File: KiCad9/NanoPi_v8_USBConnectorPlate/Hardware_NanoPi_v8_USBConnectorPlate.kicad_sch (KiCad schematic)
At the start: 30 parts, among them J1 Conn_01x02, J10 Conn_01x04, J11 Conn_01x02, J12 Conn_01x02, J2 USB_Host_Data_02x02, J3 USB_Host_Data_02x02, J4 USB_Power_02x02, J5 Conn_01x03, J6 Conn_01x09, J8 Conn_01x09, U1 USBLC6-2P6, U2 USBLC6-2P6, U3 USBLC6-2P6

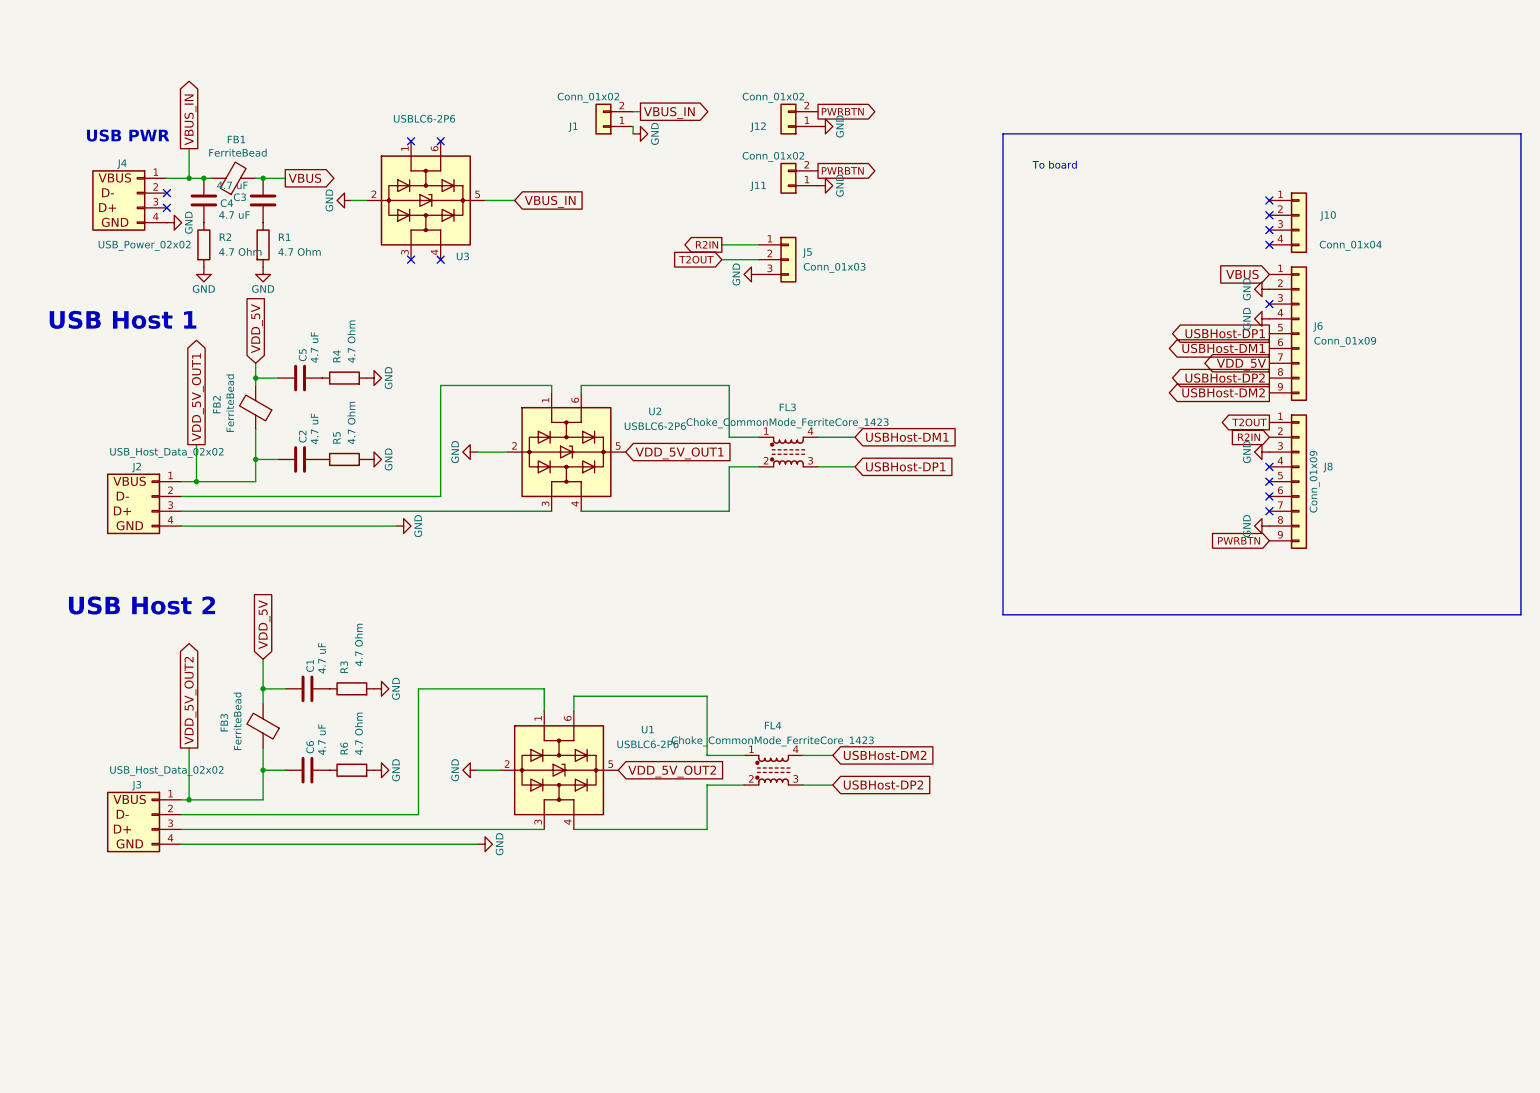
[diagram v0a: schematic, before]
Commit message: add ethernet etc
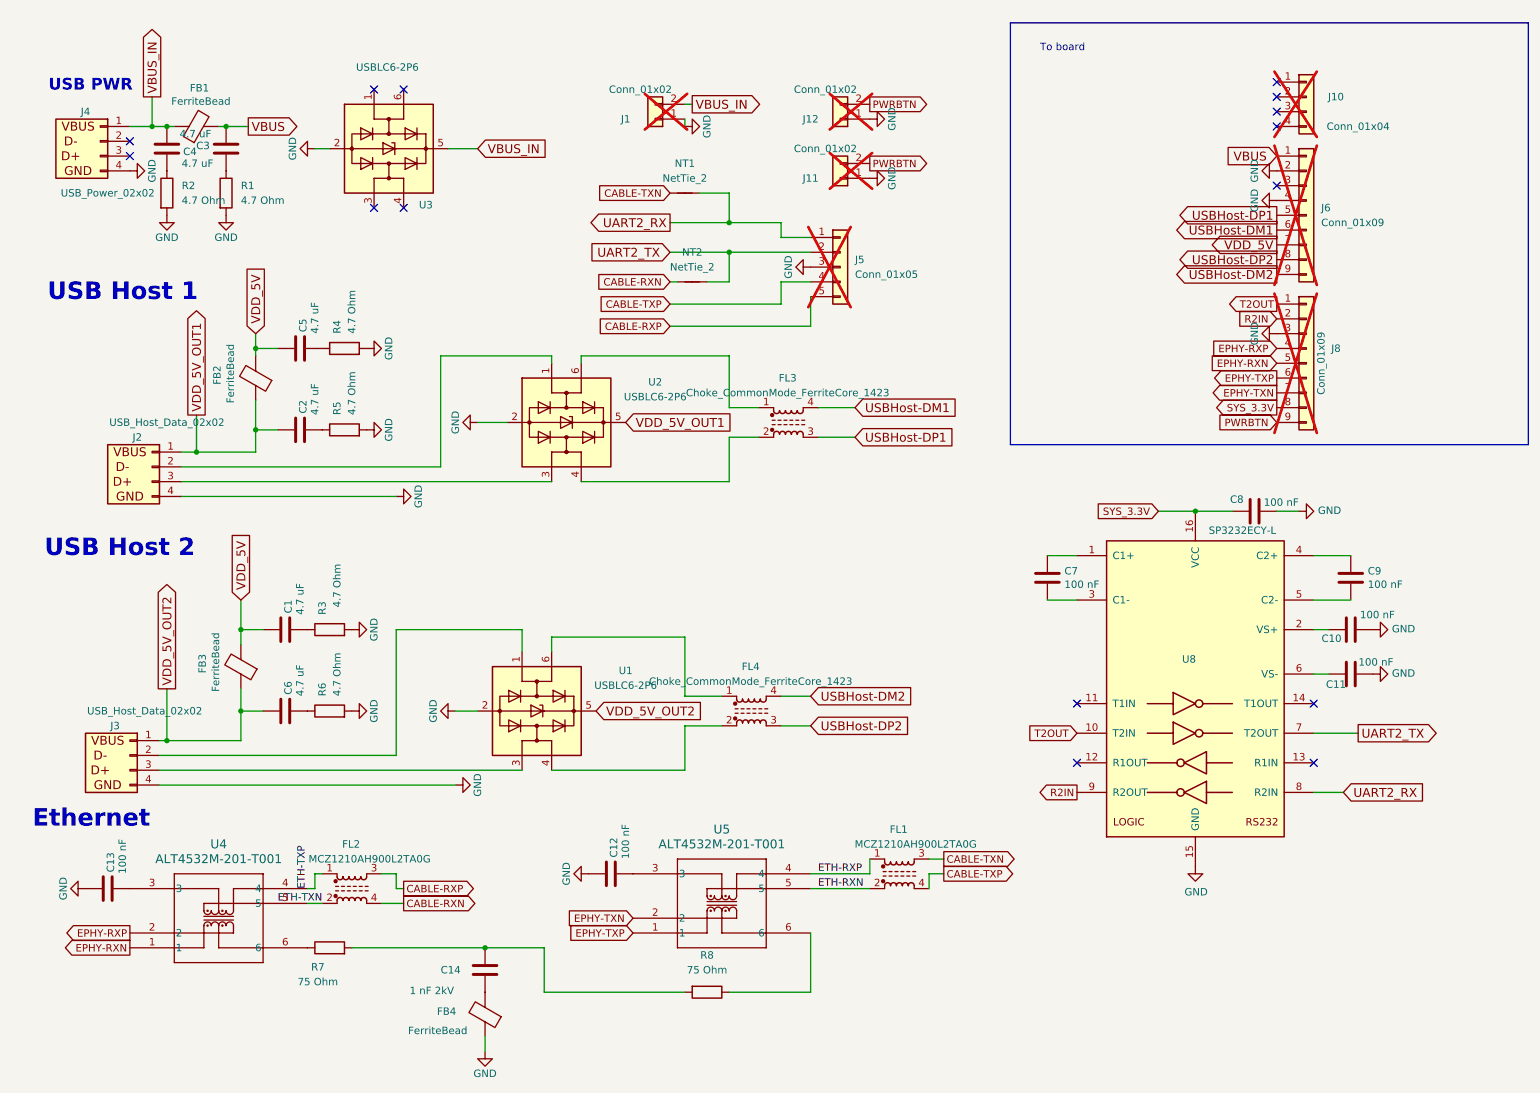
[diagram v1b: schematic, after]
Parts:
- removed J5: Conn_01x03, WiRoc:SerialConnPads3Pin, symbol Connector_Generic:Conn_01x03
- added C10, C11, C12, C13, C7, C8, C9: 100 nF, Capacitor_SMD:C_0402_1005Metric, symbol Device:C
- added C14: 1 nF 2kV, Capacitor_SMD:C_1206_3216Metric, symbol Device:C
- added FB4: FerriteBead, Inductor_SMD:L_1206_3216Metric, symbol Device:FerriteBead
- added FL1, FL2: MCZ1210AH900L2TA0G, WiRoc:MCZ1210AH_L2_TDK, symbol Filter:Choke_CommonMode_FerriteCore_1324
- added J5: Conn_01x05, WiRoc:SerialAndEthConnPads4Pin, symbol Connector_Generic:Conn_01x05
- added NT1, NT2: NetTie_2, WiRoc:NetTie-2_SMD_Pad0.3mm, symbol Device:NetTie_2
- added R7, R8: 75 Ohm, Resistor_SMD:R_0603_1608Metric, symbol Device:R
- added U4, U5: ALT4532M-201-T001, WiRoc:ALT4532M_TDK, symbol ALT4532M:ALT4532M-201-T001
- added U8: SP3232ECY-L, WiRoc:TSSOP-16_4.4x5mm_P0.65mm_PartOfSilkscreenRemoved, symbol Interface_UART:MAX3232
- C1, C2, C3, C4, C5, C6, R1, R2, R3, R4, R5, R6: JLCPCBBasic (none) -> YES
- FB1, FB2, FB3, FL3, FL4: JLCPCBBasic (none) -> NO
- J1, J10, J11, J12, J6, J8: now not fitted
- U1, U2, U3: JLCPCBBasic (none) -> NO; LCSC (none) -> C15999; LCSC Part # (none) -> C15999
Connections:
- net GND: now also C10.1, C11.1, C12.1, C13.1, C8.1, FB4.1, J5.3 (Pin_3), U8.15 (GND); no longer J8.8 (Pin_8)
- net R2IN: now also U8.9 (R2OUT)
- net T2OUT: now also U8.10 (T2IN)
- net EPHY-RXP: now reaches J8.4 (Pin_4)
- net EPHY-RXP: now also U4.2
- net EPHY-RXN: now reaches J8.5 (Pin_5)
- net EPHY-RXN: now also U4.1
- net EPHY-TXP: now reaches J8.6 (Pin_6)
- net EPHY-TXP: now also U5.1
- net EPHY-TXN: now reaches J8.7 (Pin_7)
- net EPHY-TXN: now also U5.2
- new net: C13.2, U4.3
- new net: R7.1, U4.6
- new net: C11.2, U8.6 (VS-)
- new net: C14.1, R7.2, R8.2
- new net: C14.2, FB4.2
- new net: C9.1, U8.4 (C2+)
- new net: C9.2, U8.5 (C2-)
- new net: C7.1, U8.1 (C1+)
- new net: C7.2, U8.3 (C1-)
- new net: C10.2, U8.2 (VS+)
- new net: C12.2, U5.3
- new net: R8.1, U5.6
- new net CABLE-RXN: FL2.4, NT2.1
- new net CABLE-RXP: FL2.3, J5.5 (Pin_5)
- new net CABLE-TXN: FL1.3, NT1.1
- new net CABLE-TXP: FL1.4, J5.4 (Pin_4)
- new net ETH-RXN: FL1.2, U5.5
- new net ETH-RXP: FL1.1, U5.4
- new net ETH-TXN: FL2.2, U4.5
- new net ETH-TXP: FL2.1, U4.4
- new net SYS_3.3V: C8.2, J8.8 (Pin_8), U8.16 (VCC)
- new net UART2_RX: J5.1 (Pin_1), NT1.2, U8.8 (R2IN)
- new net UART2_TX: J5.2 (Pin_2), NT2.2, U8.7 (T2OUT)
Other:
- note added: "Ethernet"
- moved on the sheet: C1, C2, C3, C4, C5, C6, FB1, FB2, FB3, FL3, FL4, J2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
